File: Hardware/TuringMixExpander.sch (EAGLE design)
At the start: 46 parts, among them IC1 TL074P, IC2 TL072P

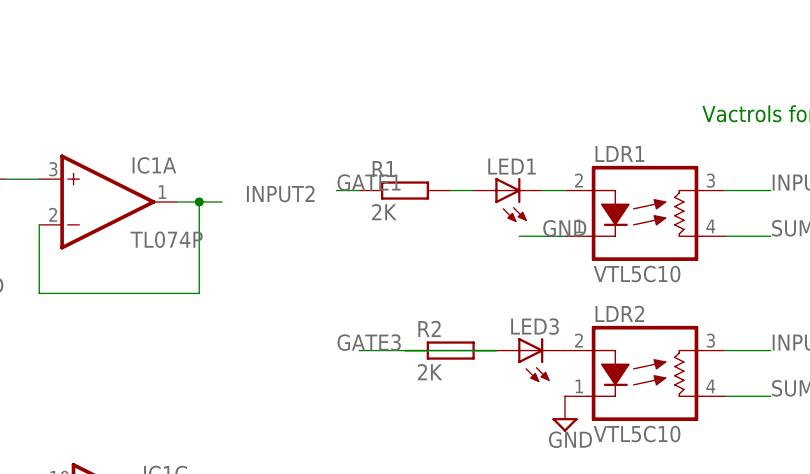
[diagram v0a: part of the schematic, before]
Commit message: New resistor grid
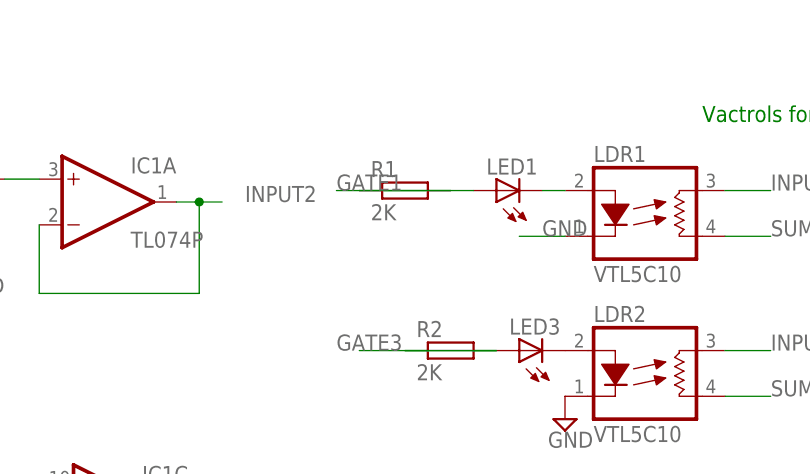
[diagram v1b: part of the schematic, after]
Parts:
- R1, R10, R11, R12, R2, R3, R4, R5, R6, R7, R8, R9: device TomW:R-EU_0207/10 -> TomW:R-EU_0207/7
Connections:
- net GATE1: now also R1.2; no longer R1.1
- net GND: now also LDR1.LED-, LDR2.LED-, LDR3.LED-, LDR4.LED-, LDR5.LED-, LDR6.LED-, LDR7.LED-, LDR8.LED-; no longer LDR1.C, LDR2.C, LDR3.C, LDR4.C, LDR5.C, LDR6.C, LDR7.C, LDR8.C
- net INPUT1: now also LDR1.RES1, LDR5.RES1; no longer LDR1.L1, LDR5.L1
- net INPUT2: now also LDR2.RES1, LDR6.RES1; no longer LDR2.L1, LDR6.L1
- net INPUT3: now also LDR3.RES1, LDR7.RES1; no longer LDR3.L1, LDR7.L1
- net INPUT4: now also LDR4.RES1, LDR8.RES1; no longer LDR4.L1, LDR8.L1
- net N$14: now also LDR1.LED+; no longer LDR1.A
- net N$15: now also LDR2.LED+; no longer LDR2.A
- net N$16: now also LDR3.LED+; no longer LDR3.A
- net N$17: now also LDR4.LED+; no longer LDR4.A
- net N$18: now also LDR5.LED+; no longer LDR5.A
- net N$19: now also LDR6.LED+; no longer LDR6.A
- net N$20: now also LDR7.LED+; no longer LDR7.A
- net N$21: now also LDR8.LED+; no longer LDR8.A
- net N$25: now also R1.1; no longer R1.2
- net SUML: now also LDR1.RES2, LDR2.RES2, LDR3.RES2, LDR4.RES2; no longer LDR1.L2, LDR2.L2, LDR3.L2, LDR4.L2
- net SUMR: now also LDR5.RES2, LDR6.RES2, LDR7.RES2, LDR8.RES2; no longer LDR5.L2, LDR6.L2, LDR7.L2, LDR8.L2

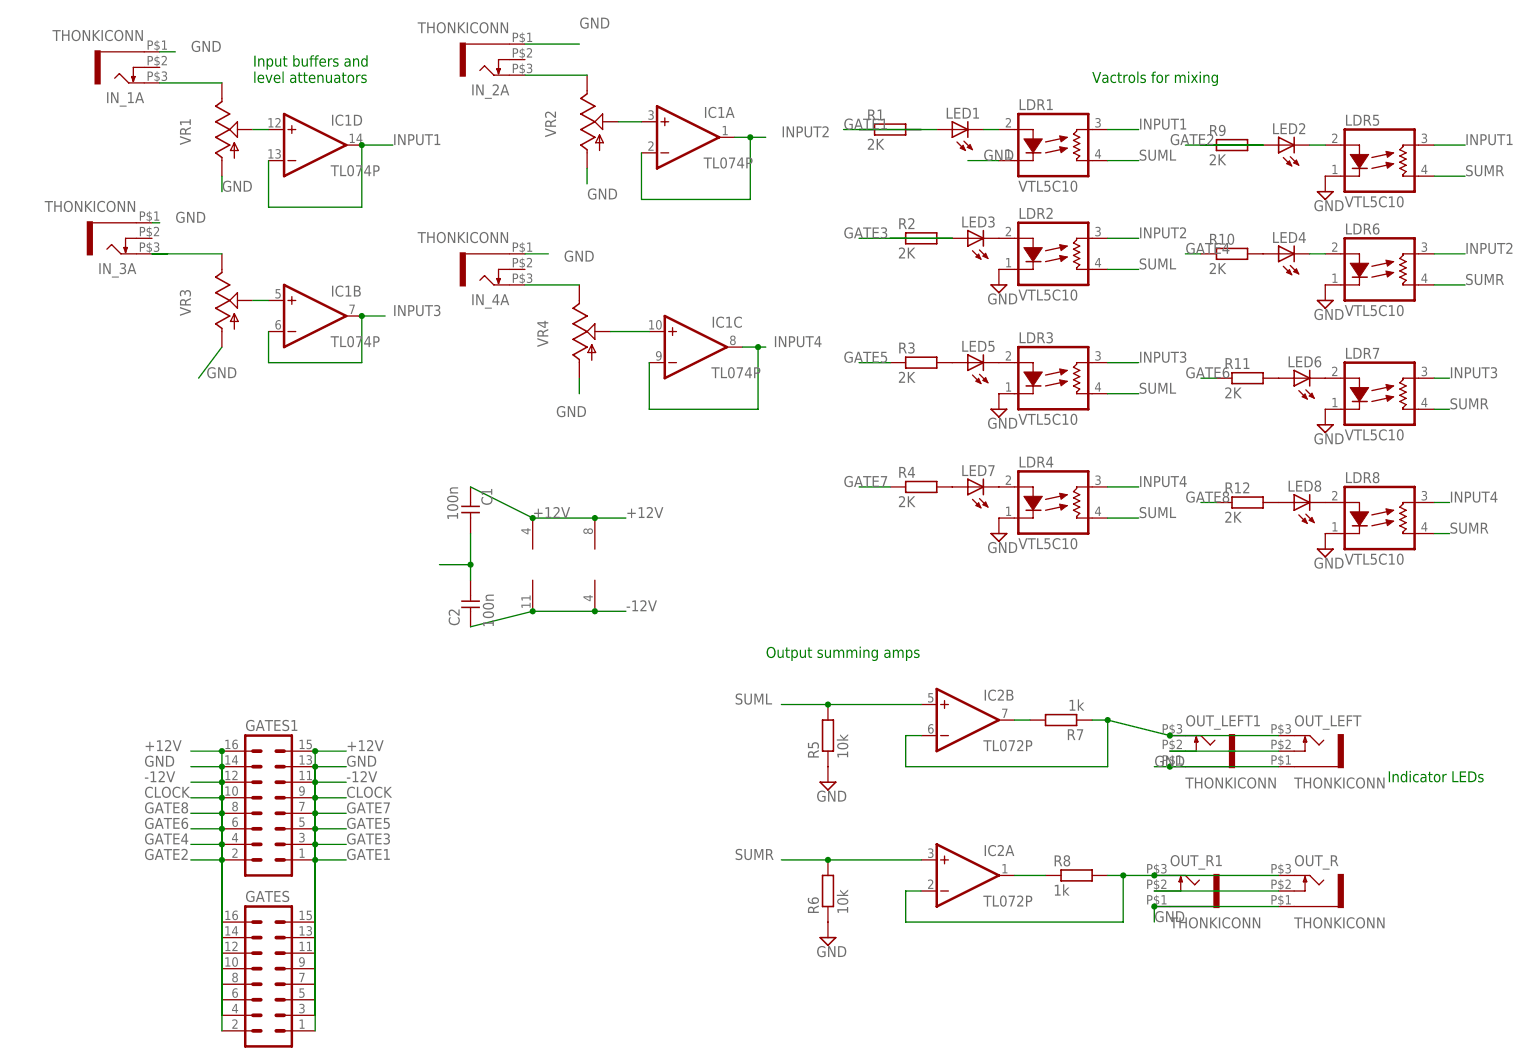
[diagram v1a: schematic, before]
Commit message: PCB work
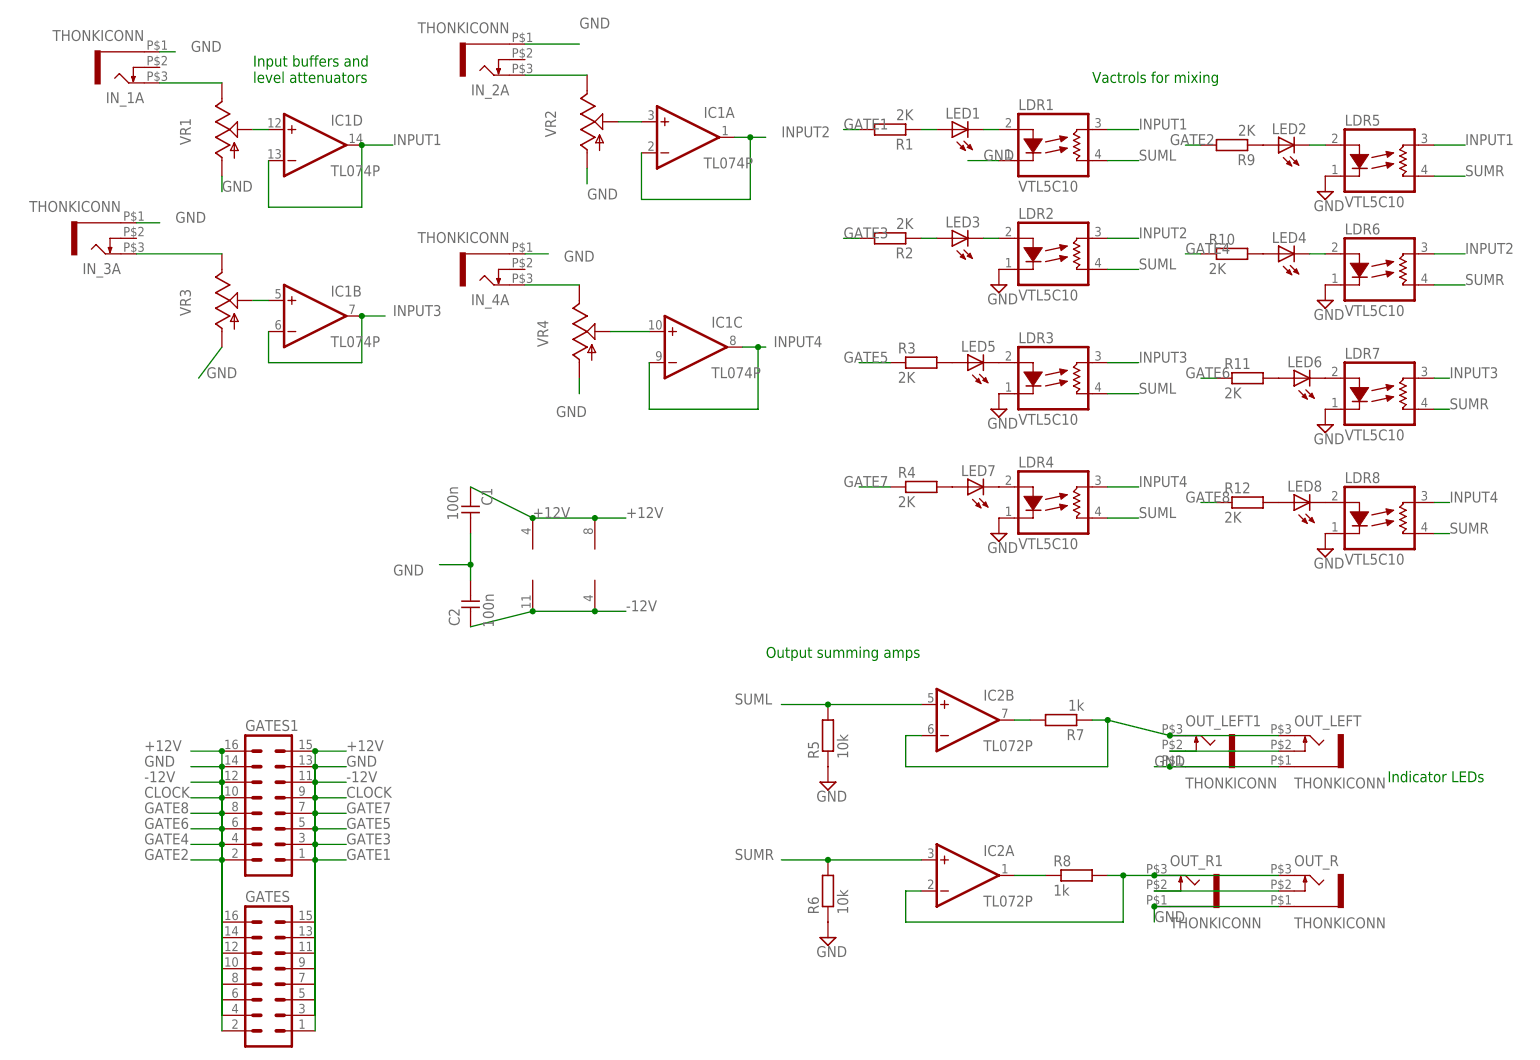
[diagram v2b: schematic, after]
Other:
- moved on the sheet: IN_3A, LED3, R1, R2, R9
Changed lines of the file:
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@@
 <instance part="IN_1A" gate="G$1" x="17.78" y="167.64" rot="R180"/>
 <instance part="IN_2A" gate="G$1" x="77.47" y="168.91" rot="R180"/>
-<instance part="IN_3A" gate="G$1" x="16.51" y="139.7" rot="R180"/>
+<instance part="IN_3A" gate="G$1" x="13.97" y="139.7" rot="R180"/>
 <instance part="IN_4A" gate="G$1" x="77.47" y="134.62" rot="R180"/>
 <instance part="IC1" gate="D" x="48.26" y="154.94"/>
@@
 <instance part="LED1" gate="G$1" x="152.4" y="157.48" rot="R90"/>
 <instance part="LED2" gate="G$1" x="205.74" y="154.94" rot="R90"/>
-<instance part="LED3" gate="G$1" x="154.94" y="139.7" rot="R90"/>
+<instance part="LED3" gate="G$1" x="152.4" y="139.7" rot="R90"/>
 <instance part="LED4" gate="G$1" x="205.74" y="137.16" rot="R90"/>
 <instance part="LED5" gate="G$1" x="154.94" y="119.38" rot="R90"/>
@@
 <instance part="FRAME1" gate="G$1" x="0" y="0"/>
 <instance part="GATES1" gate="G$1" x="40.64" y="45.72"/>
-<instance part="R1" gate="G$1" x="142.24" y="157.48"/>
+<instance part="R1" gate="G$1" x="142.24" y="157.48" rot="R180"/>
 <instance part="C1" gate="G$1" x="73.66" y="93.98" rot="R180"/>
 <instance part="C2" gate="G$1" x="73.66" y="81.28"/>
@@
 <instance part="SUPPLY8" gate="GND" x="213.36" y="129.54"/>
 <instance part="SUPPLY9" gate="GND" x="213.36" y="147.32"/>
-<instance part="R2" gate="G$1" x="147.32" y="139.7"/>
+<instance part="R2" gate="G$1" x="142.24" y="139.7" rot="R180"/>
 <instance part="R3" gate="G$1" x="147.32" y="119.38"/>
 <instance part="R4" gate="G$1" x="147.32" y="99.06"/>
-<instance part="R9" gate="G$1" x="198.12" y="154.94"/>
+<instance part="R9" gate="G$1" x="198.12" y="154.94" rot="R180"/>
 <instance part="R10" gate="G$1" x="198.12" y="137.16"/>
 <instance part="R11" gate="G$1" x="200.66" y="116.84"/>
@@
 <segment>
 <pinref part="IN_3A" gate="G$1" pin="5"/>
-<wire x1="22.86" y1="142.24" x2="21.59" y2="142.24" width="0.1524" layer="91"/>
+<wire x1="22.86" y1="142.24" x2="19.05" y2="142.24" width="0.1524" layer="91"/>
 <label x="25.4" y="142.24" size="1.778" layer="95"/>
 </segment>
@@
 <wire x1="68.58" y1="86.36" x2="73.66" y2="86.36" width="0.1524" layer="91"/>
 <junction x="73.66" y="86.36"/>
+<label x="66.04" y="86.36" size="1.778" layer="95" rot="R180"/>
 </segment>
 <segment>
@@
 <segment>
 <pinref part="R1" gate="G$1" pin="2"/>
-<wire x1="134.62" y1="157.48" x2="147.32" y2="157.48" width="0.1524" layer="91"/>
+<wire x1="134.62" y1="157.48" x2="137.16" y2="157.48" width="0.1524" layer="91"/>
 <label x="134.62" y="157.48" size="1.778" layer="95"/>
 </segment>
@@
 <segment>
 <pinref part="R9" gate="G$1" pin="2"/>
-<wire x1="190.5" y1="154.94" x2="203.2" y2="154.94" width="0.1524" layer="91"/>
+<wire x1="190.5" y1="154.94" x2="193.04" y2="154.94" width="0.1524" layer="91"/>
 <label x="187.96" y="154.94" size="1.778" layer="95"/>
 </segment>
@@
 <segment>
 <pinref part="R2" gate="G$1" pin="2"/>
-<wire x1="137.16" y1="139.7" x2="152.4" y2="139.7" width="0.1524" layer="91"/>
+<wire x1="134.62" y1="139.7" x2="137.16" y2="139.7" width="0.1524" layer="91"/>
 <label x="134.62" y="139.7" size="1.778" layer="95"/>
 </segment>
@@
 <segment>
 <pinref part="VR3" gate="G$1" pin="E"/>
-<wire x1="33.02" y1="137.16" x2="21.59" y2="137.16" width="0.1524" layer="91"/>
+<wire x1="33.02" y1="137.16" x2="19.05" y2="137.16" width="0.1524" layer="91"/>
 <pinref part="IN_3A" gate="G$1" pin="3"/>
-<wire x1="24.13" y1="137.16" x2="21.59" y2="137.16" width="0.1524" layer="91"/>
 </segment>
 </net>
@@
 <pinref part="LDR2" gate="G$1" pin="LED+"/>
 <pinref part="LED3" gate="G$1" pin="C"/>
+<wire x1="157.48" y1="139.7" x2="160.02" y2="139.7" width="0.1524" layer="91"/>
 </segment>
 </net>
@@
 <pinref part="LED1" gate="G$1" pin="A"/>
 <pinref part="R1" gate="G$1" pin="1"/>
-<wire x1="137.16" y1="157.48" x2="149.86" y2="157.48" width="0.1524" layer="91"/>
+<wire x1="147.32" y1="157.48" x2="149.86" y2="157.48" width="0.1524" layer="91"/>
 </segment>
 </net>
@@
 <pinref part="LED3" gate="G$1" pin="A"/>
 <pinref part="R2" gate="G$1" pin="1"/>
-<wire x1="152.4" y1="139.7" x2="142.24" y2="139.7" width="0.1524" layer="91"/>
+<wire x1="147.32" y1="139.7" x2="149.86" y2="139.7" width="0.1524" layer="91"/>
 </segment>
 </net>
@@
 <pinref part="LED2" gate="G$1" pin="A"/>
 <pinref part="R9" gate="G$1" pin="1"/>
-<wire x1="203.2" y1="154.94" x2="193.04" y2="154.94" width="0.1524" layer="91"/>
 </segment>
 </net>
@@
 </sheet>
 </sheets>
+<errors>
+</errors>
 </schematic>
 </drawing>
